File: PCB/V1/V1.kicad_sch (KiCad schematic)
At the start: 33 parts, among them J2 USB3131-30-0230-A_REVB, J4 Programmer, J5 Conn_02x06_Odd_Even, J6 Conn_02x06_Odd_Even, J7 RESET, J8 RESET, U2 MDBT50Q-1MV2, Y1 32.768kHz

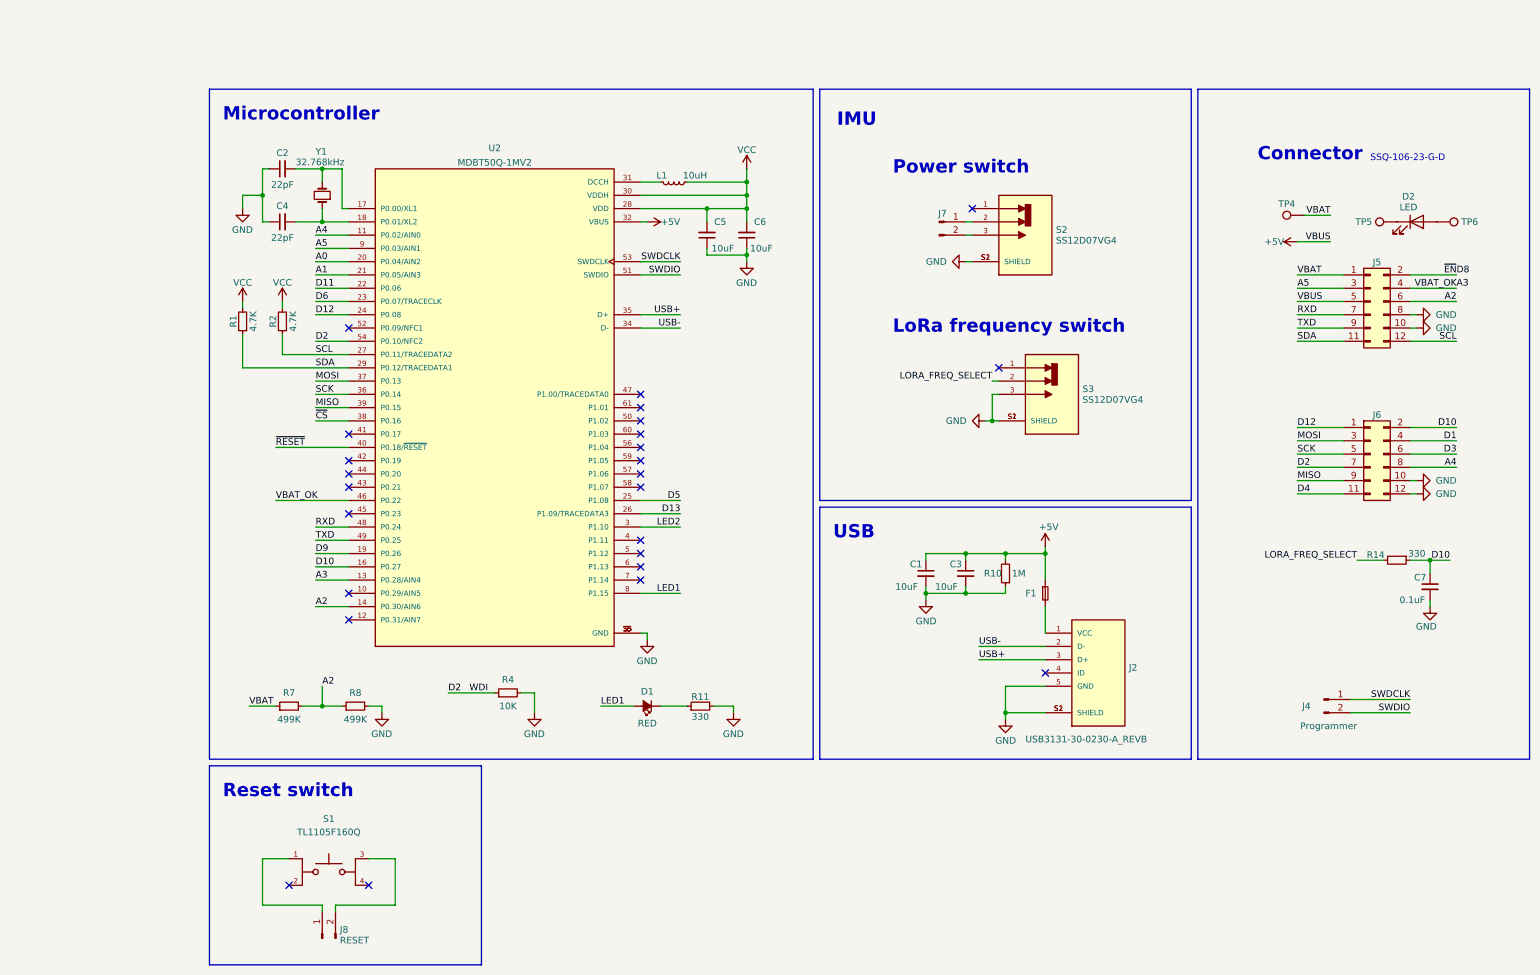
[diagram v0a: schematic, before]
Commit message: udated by FZ
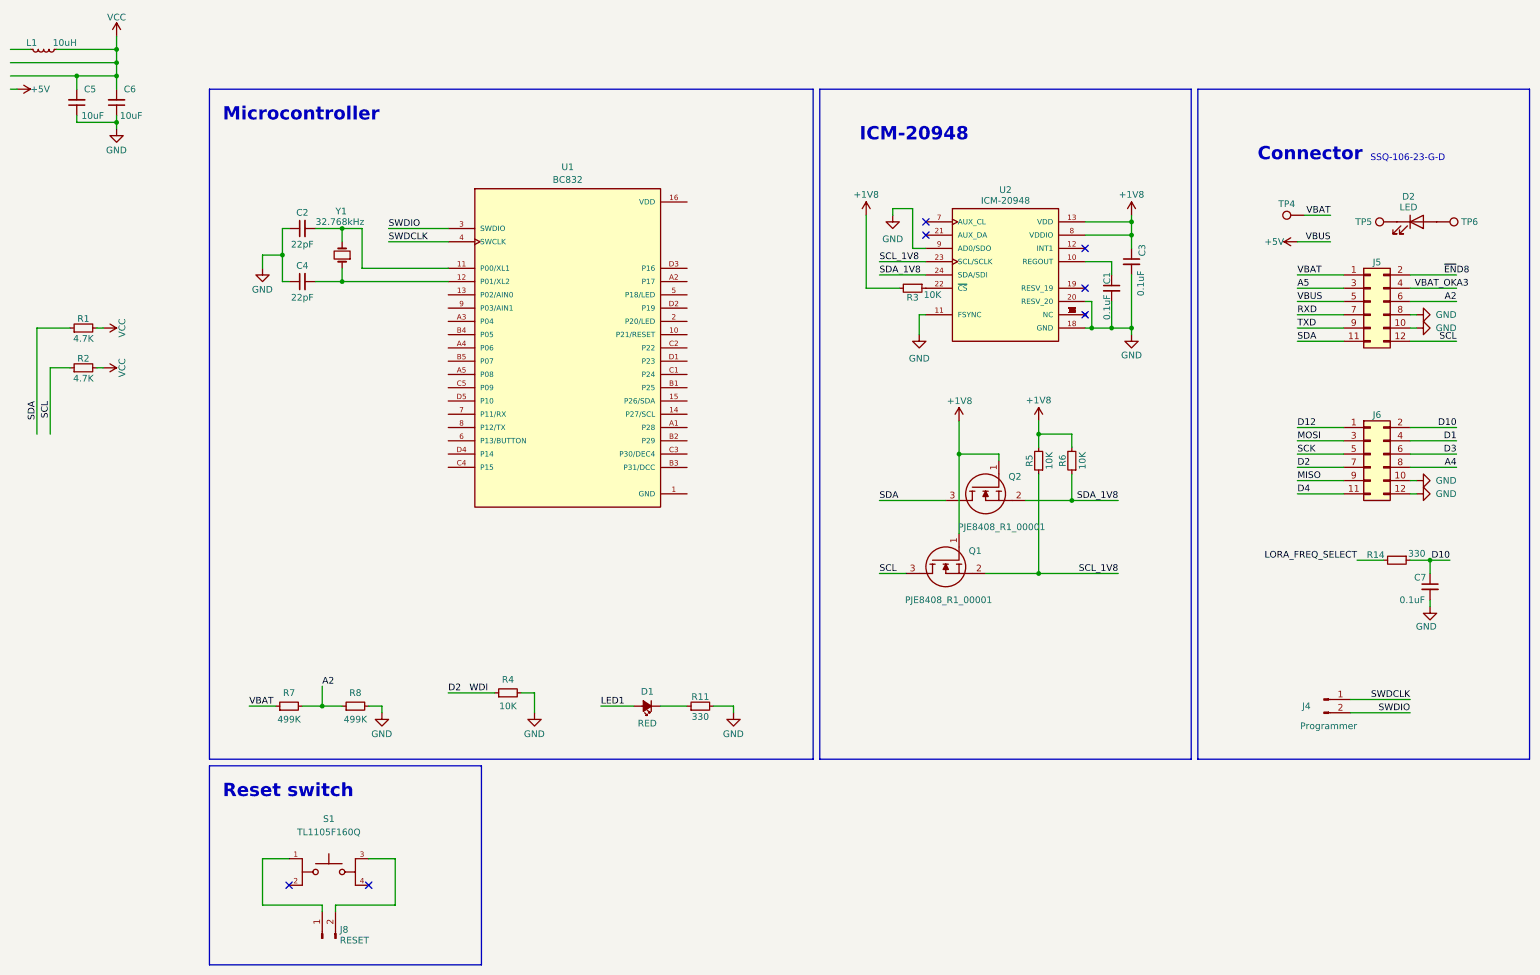
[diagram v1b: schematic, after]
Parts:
- removed F1: Fuse_Small, Fuse:Fuse_1206_3216Metric_Pad1.42x1.75mm_HandSolder, symbol Device:Fuse_Small
- removed J2: USB3131-30-0230-A_REVB, Mylib:GCT_USB3131-30-0230-A_REVB, symbol USB3131-30-0230-A_REVB:USB3131-30-0230-A_REVB
- removed J7: RESET, Connector_PinHeader_2.00mm:PinHeader_1x02_P2.00mm_Vertical, symbol Connector:Conn_01x02_Pin
- removed R10: 1M, Resistor_SMD:R_0603_1608Metric_Pad0.98x0.95mm_HandSolder, symbol Device:R_Small
- removed S2, S3: SS12D07VG4, Mylib:SW_SS12D07VG4, symbol SS12D07VG4:SS12D07VG4
- removed U2: MDBT50Q-1MV2, Mylib:XCVR_MDBT50Q-1MV2, symbol MDBT50Q-1MV2:MDBT50Q-1MV2
- added Q1, Q2: PJE8408_R1_00001, SamacSys_Parts:SOTFL50P160X60-3N, symbol SamacSys_Parts:PJE8408_R1_00001
- added R3, R5, R6: 10K, Resistor_SMD:R_0402_1005Metric_Pad0.72x0.64mm_HandSolder, symbol Device:R_Small
- added U1: BC832, XCVR_BC832, symbol BC832:BC832
- added U2: ICM-20948, Sensor_Motion:InvenSense_QFN-24_3x3mm_P0.4mm, symbol ICM-20948:ICM-20948
- C1, C3: value 10uF -> 0.1uF; footprint Capacitor_SMD:C_1206_3216Metric_Pad1.33x1.80mm_HandSolder -> Capacitor_SMD:C_0402_1005Metric_Pad0.74x0.62mm_HandSolder
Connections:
- net +5V: no longer C1.1, C3.1
- net GND: now also U2.11 (FSYNC), U2.18 (GND), U2.20 (RESV_20), U2.9 (AD0/SDO)
- net SCL: now also Q1.3
- net SDA: now also Q2.3
- net SWDCLK: now also U1.4 (SWCLK)
- net SWDIO: now also U1.3 (SWDIO)
- net at C2.2, Y1.2: now also U1.11 (P00/XL1)
- net at C4.2, Y1.1: now also U1.12 (P01/XL2)
- new net: R3.1, U2.22 (~{CS})
- new net: C1.1, U2.10 (REGOUT)
- new net: U2.1 (NC), U2.14 (NC), U2.15 (NC), U2.16 (NC), U2.17 (NC), U2.2 (NC), U2.3 (NC), U2.4 (NC), U2.5 (NC), U2.6 (NC)
- new net +1V8: C3.1, Q1.1, Q2.1, R3.2, R5.2, R6.2, U2.13 (VDD), U2.8 (VDDIO)
- new net SCL_1V8: Q1.2, R5.1, U2.23 (SCL/SCLK)
- new net SDA_1V8: Q2.2, R6.1, U2.24 (SDA/SDI)
- no-connect marks 25 -> 7
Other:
- note added: "ICM-20948"
- note removed: "IMU"
- note removed: "LoRa frequency switch"
- note removed: "Power switch"
- note removed: "USB"
- moved on the sheet: C2, C4, C5, C6, L1, R1, R2, Y1
